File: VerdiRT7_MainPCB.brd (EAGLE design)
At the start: 146 x 66 mm, 188 parts, among them J1 RECEPT_SMD_5-2, J13 DF58_2P, J15 503480_0400, J16 503480_0600, J2 RECEPT_SMD_5-2, J4 MOLEX_105027, J6 52559-0652, J7 503480_1400, J8 BM02B-SRSS-TB, Q1 SIZ322DT, Q2 SIZ322DT, Q3 SIZ322DT, Q5 SIZ322DT, Q6 SIZ322DT, Q7 SI7615ADN, Q8 SIZ322DT, SW1 AYZ0102AGRLC, SW3 SKRH, SW4 TACT_SWITCHO, U10 RT9625A, U13 MCP1416, U14 MCP1416, U15 MCP1416, U16 MCP6001, U17 MCP6001, U18 RT9625A, U19 ICM-20602, U3 7408_3, U4 RT9625A, U5 MCP6001, U6 MCP1416, U7 7408_3, U8 7408_3, U9 MCP6001, X1 NX3225

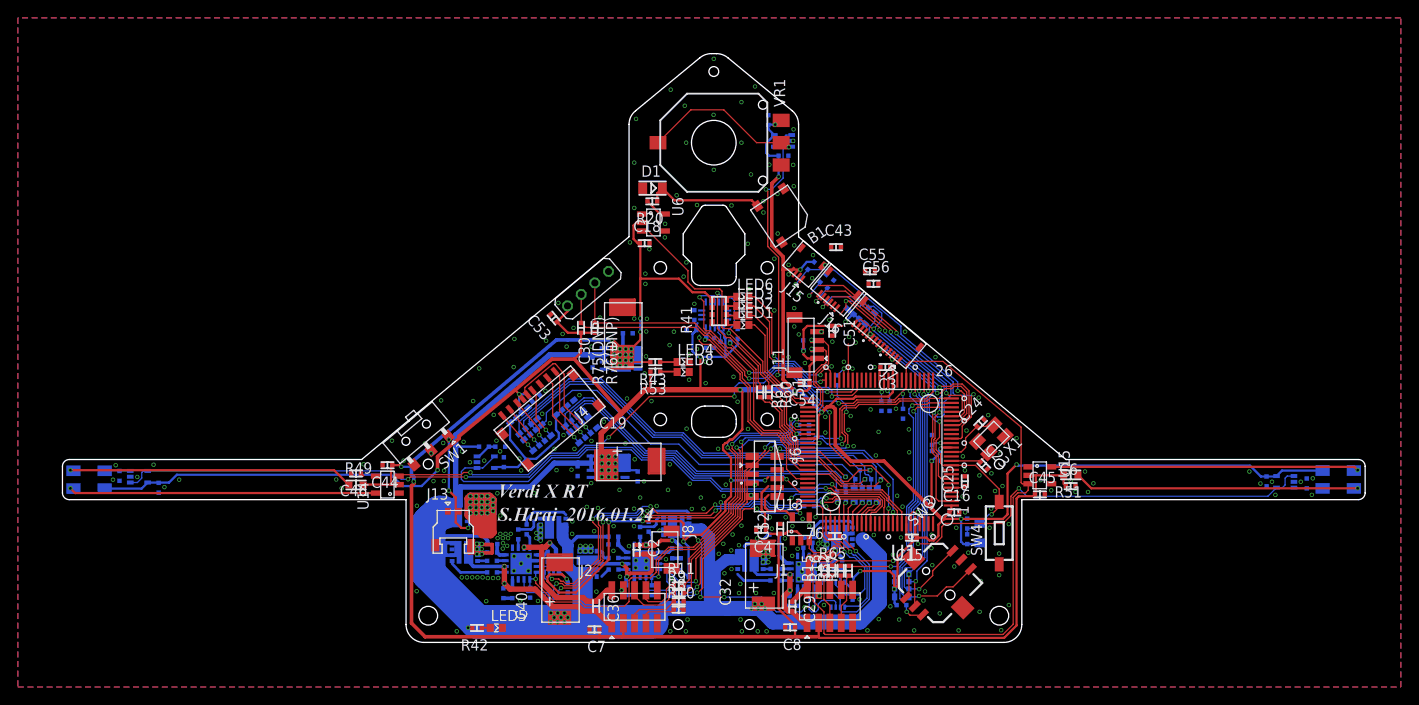
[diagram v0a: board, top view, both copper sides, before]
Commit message: updated: DRC 終了
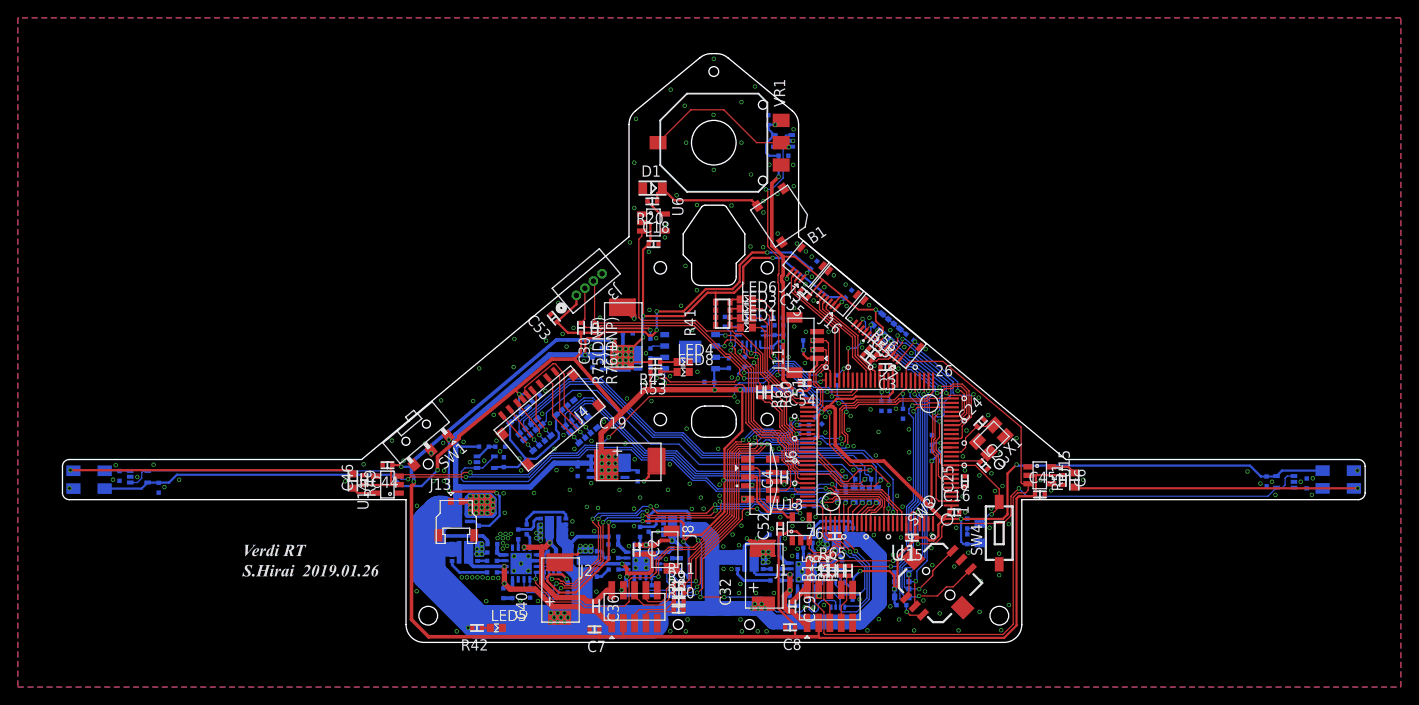
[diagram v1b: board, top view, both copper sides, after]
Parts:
- removed CH1: 1X4P, pin_header_2mm:1X4P
- added C57: 10V 0.1u, capacitor:1005
- added J3: DF13-4P-1.25DSA, Hirose_DF:DF13_4P_TH
- added R64, R74: 100k, resistor:1005
- added R75: 22, resistor:1005
- added U2: MR20H40, Memory:8DFN
- moved R54 13.7 mm to (95.0, 34.2), turned to 40 degrees
- moved C10 10.3 mm to (80.8, 35.0), turned to 90 degrees
- moved C51 10.2 mm to (84.7, 24.9), flipped to the bottom, turned to 225 degrees
- moved R55 10.2 mm to (90.2, 31.9), flipped to the top, turned to 320 degrees
- moved C42 9.95 mm to (80.1, 33.1), turned to 180 degrees
- moved R56 8.92 mm to (90.8, 32.6), flipped to the top, turned to 320 degrees
- moved C55 7.73 mm to (83.2, 39.1), turned to 140 degrees
- moved C26 7.70 mm to (80.2, 36.4), turned to 180 degrees
- moved C4 6.42 mm to (80.9, 18.5), turned to 90 degrees
- moved U19 4.48 mm to (77.2, 34.9), turned to 90 degrees
- moved C21 4.16 mm to (79.8, 35.0)
- moved R57 3.37 mm to (92.4, 35.4), turned to 40 degrees
- moved C43 3.20 mm to (84.2, 42.3), flipped to the bottom, turned to 130 degrees
- moved R3 3.17 mm to (74.2, 35.9), turned to 270 degrees
- moved R63 3.11 mm to (76.5, 31.4), turned to 270 degrees
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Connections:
- new net N$16: R64.P$1, U2.7
- new net N$21: R74.P$1, U2.3
- new net N$45: R75.P$2, U2.2
- net +3V3: now also C57.P$1, J3.1, R64.P$2, R74.P$2, U2.8; no longer CH1.1
- net GND: now also C57.P$2, J13.1, J3.4, Q1.5, Q1.6, Q1.7, Q5.5, Q5.6, Q5.7, Q6.5, Q6.6, Q6.7, U2.4, U2.PAD; no longer CH1.4, J13.2
- net RXD2_BTM: now also J3.3; no longer CH1.3
- net SPI_CS1: now also U2.1
- net SPI_MISO: now also R75.P$1
- net SPI_MOSI: now also U2.5
- net SPI_SCK: now also U2.6
- net TXD2_BTM: now also J3.2; no longer CH1.2
- net VCC: now also J13.2; no longer J13.1
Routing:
- net +8V: track 224.8 -> 268.8 mm, vias 15 -> 20
- net N$54: track 35.6 -> 2.85 mm, vias 1 -> 0
- net N$5: track 34.5 -> 2.80 mm, vias 1 -> 0
- net SPI_CS1: track 0.00 -> 26.1 mm, vias 0 -> 1
- net +5V: track 244.2 -> 267.0 mm, vias 20 -> 22
- net +3V3: track 457.0 -> 476.4 mm, vias 35 -> 36
- net TCK: track 29.8 -> 15.4 mm
- net IO_SPARE4: track 0.00 -> 14.3 mm
- net VCC: track 43.5 -> 29.4 mm
- net IO_SPARE3: track 0.00 -> 14.1 mm
- net TDO: track 27.4 -> 15.2 mm, vias 3 -> 2
- net IO_SPARE2: track 0.00 -> 11.8 mm
- net IO_SPARE1: track 0.00 -> 11.6 mm
- net IO_SPARE0: track 0.00 -> 11.4 mm
- net SPI_MISO: track 23.3 -> 33.4 mm, vias 2 -> 4
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- removed copper zone on layer 1, net VCC

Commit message: updated: リナンバー完了，BOM 完了
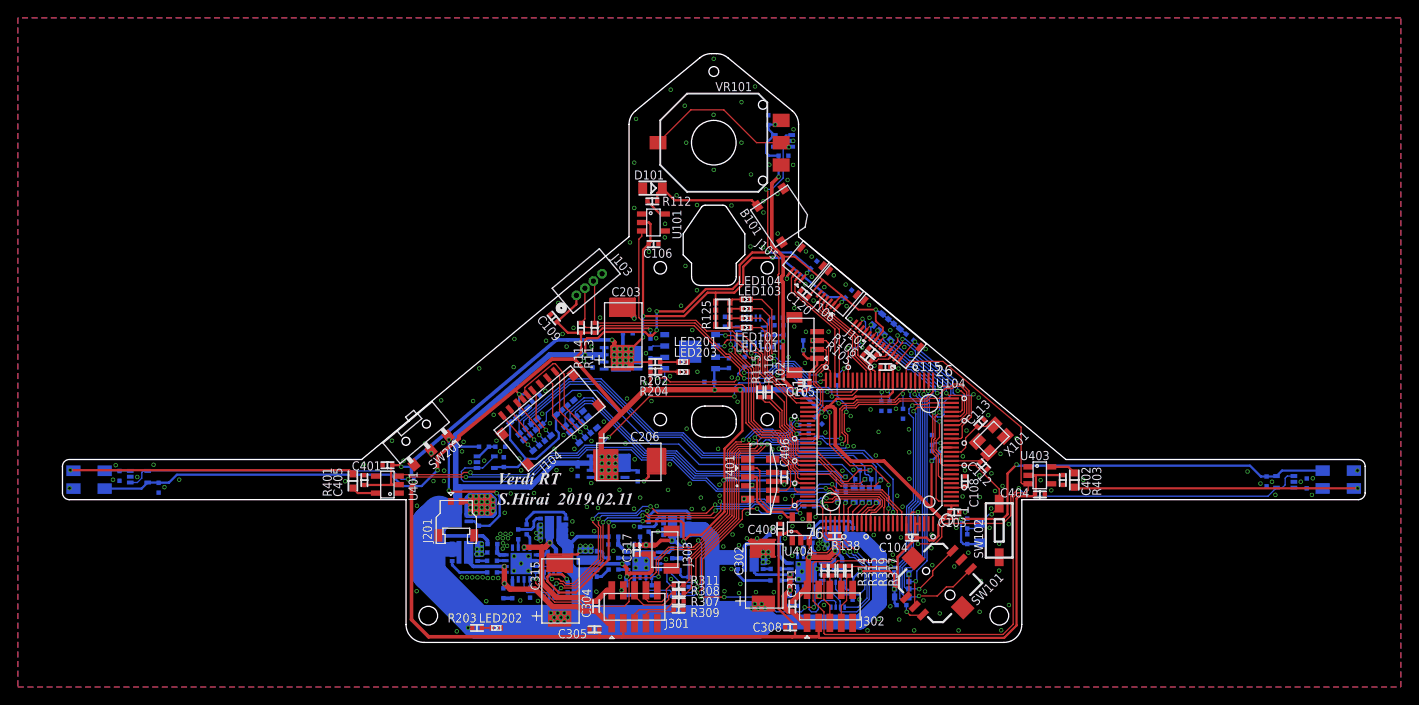
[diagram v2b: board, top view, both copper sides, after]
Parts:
- removed C19, C30: 16V33u, capacitor:EEFCX_7343
- removed C32, C40: 16V 33u, capacitor:EEFCX_7343
- removed LED1, LED2, LED3, LED4, LED5, LED6, LED8: (no value), led:1608-OLI
- removed Q7: SI7615ADN, MOSFET:POWERPAK1212-8
- removed SW4: TACT_SWITCHO, switch:TACT_SWITCH-OLI
- removed U3, U7, U8: 7408_3, 74xx-eu:VSSOP8
- added C203, C206, C302, C315: EEF-CS1C330R, capacitor:EEFC_7343
- added LED101, LED102, LED103, LED104: APHHS1005QBC/D, LED:1005
- added LED201, LED203: APHHS1005SYCK, LED:1005
- added LED202: APHHS1005ZGC, LED:1005
- added Q201: SISA01DN-T1-GE3, MOSFET:POWERPAK1212-8
- added SW102: SKQYACE010, switch:SKQYA
- added U301, U303, U305: 74LVC2G08DC, 74xx-eu:VSSOP8
- B101: value SMT-0540-S-R -> SMT-0540-T-7-R
- J102: value (none) -> BM04B-SRSS-TB(LF)(SN)
- J104: value MOLEX_105027 -> 1050270001
- J201: value DF58_2P -> DF58-2P-1.2V(21)
- J301, J302: value RECEPT_SMD_5-2 -> 20021321-00010C4LF
- J303: value BM02B-SRSS-TB -> BM02B-SRSS-TB(LF)(SN)
- Q301, Q302, Q303, Q304, Q305, Q306: value SIZ322DT -> SIZ322DT-T1-GE3
- R113, R114: value 20k -> 20k (DNP)
- R117, R118, R123: value 22 -> 22 (DNP)
- R140: value 100k -> 100k (DNP)
- SW101: value SKRH -> SKRHABE010
- U101, U401, U403, U404: value MCP1416 -> MCP1416T-E/OT
- U102, U103, U402, U405: value MCP6001 -> MCP6001T-I/LT
- U104: value (none) -> R5F564MLDDFP#V1-ND
- U105: value MR20H40 -> MR20H40CDF
- U201: value (none) -> TLV1117-50CDRJR
- U202: value (none) -> TLV1117-33CDRJR
- U302, U304, U306: value RT9625A -> RT9625AZQW
- VR101: value SV01 -> SV01A103AEA01
- X101: value NX3225 -> NX3225SA-12.000M-STD-CSR-1
- renumbered B1 to B101, C1 to C204, C10 to C501, C11 to C314, C12 to C201, C13 to C316, C14 to C310, C15 to C104, C16 to C103, C17 to C102, C18 to C106, C2 to C317, C20 to C313, C21 to C502, C22 to C117, C23 to C112, C24 to C113, C25 to C108, C26 to C504, C27 to C111, C28 to C309, C29 to C311, C3 to C115, C31 to C312, C33 to C303, C34 to C307, C35 to C301, C36 to C304, C37 to C205, C38 to C202, C39 to C306, C4 to C406, C41 to C114, C42 to C503, C43 to C119, C44 to C401, C45 to C404, C46 to C405, C47 to C107, C48 to C110, C49 to C403, C5 to C318, C50 to C407, C51 to C101, C52 to C408, C53 to C109, C54 to C105, C55 to C120, C56 to C118, C57 to C116, C6 to C402, C7 to C305, C8 to C308, C9 to C319, D1 to D101, D2 to D102, J1 to J302, J11 to J102, J13 to J201, J15 to J105, J16 to J106, J2 to J301, J3 to J103, J4 to J104, J6 to J401, J7 to J101, J8 to J303, PI1 to PI401, PI2 to PI402, Q1 to Q305, Q2 to Q306, Q3 to Q302, Q5 to Q301, Q6 to Q303, Q8 to Q304, R1 to R110, R10 to R309, R11 to R311, R12 to R111, R13 to R104, R14 to R107, R15 to R314, R16 to R315, R17 to R317, R18 to R136, R19 to R404, R2 to R324, R20 to R112, R21 to R109, R22 to R108, R23 to R330, R24 to R327, R25 to R329, R26 to R325, R27 to R318, R28 to R323, R29 to R331, R3 to R502, R30 to R124, R31 to R128, R32 to R319, R33 to R316, R34 to R321, R35 to R320, R36 to R322, R37 to R313, R38 to R303, R39 to R312, R4 to R326, R40 to R302, R41 to R125, R42 to R203, R43 to R202, R44 to R306, R45 to R201, R46 to R304, R47 to R310, R48 to R301, R49 to R401, R5 to R103, R50 to R402, R51 to R403, R52 to R405, R53 to R204, R54 to R101, R55 to R105, R56 to R106, R57 to R102, R58 to R120, R59 to R119, R6 to R305, R60 to R116, R61 to R115, R62 to R137, R63 to R501, R64 to R131, R65 to R138, R66 to R129, R67 to R133, R68 to R132, R69 to R135, R7 to R328, R70 to R122, R70(DNP) to R123, R71 to R121, R71(DNP) to R117, R72 to R126, R72(DNP) to R118, R73 to R127, R73_ to R139, R74 to R130, R74(DNP) to R140, R75 to R134, R75(DNP) to R114, R76(DNP) to R113, R8 to R307, R9 to R308, SW1 to SW201, SW3 to SW101, U1 to U104, U10 to U302, U11 to U201, U12 to U202, U13 to U404, U14 to U401, U15 to U403, U16 to U402, U17 to U405, U18 to U306, U19 to U501, U2 to U105, U4 to U304, U5 to U103, U6 to U101, U9 to U102, VR1 to VR101, X1 to X101
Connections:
- net AD_ASEN1 renamed AD_LINE_L_SEN
- net AD_ASEN2 renamed AD_LINE_R_SEN
- net AD_DSEN1 renamed AD_MARKER_L_SEN
- net AD_DSEN2 renamed AD_MARKER_R_SEN
- net MOTOR7 renamed DRIVE_MOTOR_EN
- net MOTOR8 renamed SENSOR_MOTOR_EN
- net TCLK1 renamed RIGHT_TCLKA
- net TCLK2 renamed RIGHT_TCLKB
- net TCLK3 renamed LEFT_TCLKC
- net TCLK4 renamed LEFT_TCLKD
- removed net MOTOR1: U104.86, U7.1
- removed net MOTOR2: U104.85, U7.6
- removed net MOTOR3: U104.78, U3.1
- removed net MOTOR4: U104.75, U3.6
- removed net MOTOR5: U104.74, U8.1
- removed net MOTOR6: U104.61, U8.6
- removed net PWM_MOTOR1: R137.P$1, U7.2, U7.5
- removed net PWM_MOTOR2: R138.P$1, U3.2, U3.5
- removed net PWM_MOTOR3: R129.P$1, U8.2, U8.5
- new net LEFT_MOTOR_CCW: U104.86, U301.1
- new net LEFT_MOTOR_CW: U104.85, U301.6
- new net LEFT_MOTOR_PWM: R137.P$1, U301.2, U301.5
- new net RIGHT_MOTOR_CCW: U104.78, U303.1
- new net RIGHT_MOTOR_CW: U104.75, U303.6
- new net RIGHT_MOTOR_PWM: R138.P$1, U303.2, U303.5
- new net SENSOR_MOTOR_CCW: U104.74, U305.1
- new net SENSOR_MOTOR_CW: U104.61, U305.6
- new net SENSOR_MOTOR_PWM: R129.P$1, U305.2, U305.5
- net +3V3: now also C206.PLUS, U301.8, U303.8, U305.8; no longer C19.PLUS, U3.8, U7.8, U8.8
- net +5V: now also C203.PLUS; no longer C30.PLUS
- net +8V: now also C302.PLUS, C315.PLUS, Q201.5, Q201.9; no longer C32.PLUS, C40.PLUS, Q7.5, Q7.9
- net GND: now also C203.MINUS, C206.MINUS, C302.MINUS, C315.MINUS, LED201.K, LED202.K, LED203.K, SW102.2, U301.4, U303.4, U305.4; no longer C19.MINUS, C30.MINUS, C32.MINUS, C40.MINUS, LED4.K, LED5.K, LED8.K, SW4.2, U3.4, U7.4, U8.4
- net LED0: now also LED101.K; no longer LED1.K
- net LED1: now also LED102.K; no longer LED2.K
- net LED2: now also LED103.K; no longer LED3.K
- net LED3: now also LED104.K; no longer LED6.K
- net N$1: now also Q201.4; no longer Q7.4
- net N$12: now also LED201.A; no longer LED4.A
- net N$3: now also LED202.A; no longer LED5.A
- net N$31: now also U303.7; no longer U3.7
- net N$33: now also U303.3; no longer U3.3
- net N$49: now also U301.7; no longer U7.7
- net N$50: now also U301.3; no longer U7.3
- net N$56: now also LED101.A; no longer LED1.A
- net N$57: now also LED102.A; no longer LED2.A
- net N$58: now also LED103.A; no longer LED3.A
- net N$59: now also LED104.A; no longer LED6.A
- net N$70: now also U305.7; no longer U8.7
- net N$71: now also U305.3; no longer U8.3
- net N$78: now also LED203.A; no longer LED8.A
- net RESET: now also SW102.1; no longer SW4.1
- net VCC: now also Q201.1; no longer Q7.1
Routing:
- net MOTOR2: track 50.3 -> 0.00 mm, vias 5 -> 0
- net LEFT_MOTOR_CW: track 0.00 -> 50.3 mm, vias 0 -> 5
- net LEFT_MOTOR_CCW: track 0.00 -> 49.5 mm, vias 0 -> 5
- net MOTOR1: track 49.4 -> 0.00 mm, vias 5 -> 0
- net SENSOR_MOTOR_PWM: track 0.00 -> 43.2 mm, vias 0 -> 4
- net PWM_MOTOR3: track 43.2 -> 0.00 mm, vias 4 -> 0
- net PWM_MOTOR1: track 40.0 -> 0.00 mm, vias 4 -> 0
- net LEFT_MOTOR_PWM: track 0.00 -> 39.4 mm, vias 0 -> 4
- net SENSOR_MOTOR_CW: track 0.00 -> 31.4 mm, vias 0 -> 3
- net MOTOR6: track 31.4 -> 0.00 mm, vias 3 -> 0
- net MOTOR5: track 22.8 -> 0.00 mm, vias 3 -> 0
- net SENSOR_MOTOR_CCW: track 0.00 -> 22.8 mm, vias 0 -> 3
- net RIGHT_MOTOR_CW: track 0.00 -> 18.2 mm, vias 0 -> 1
- net MOTOR4: track 17.9 -> 0.00 mm, vias 1 -> 0
- net RIGHT_MOTOR_PWM: track 0.00 -> 16.0 mm, vias 0 -> 1
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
